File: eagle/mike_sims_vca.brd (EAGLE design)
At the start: 100 x 80 mm, 33 parts, among them IC2 LM13700N, IC3 TL072P, Q1 2N3906

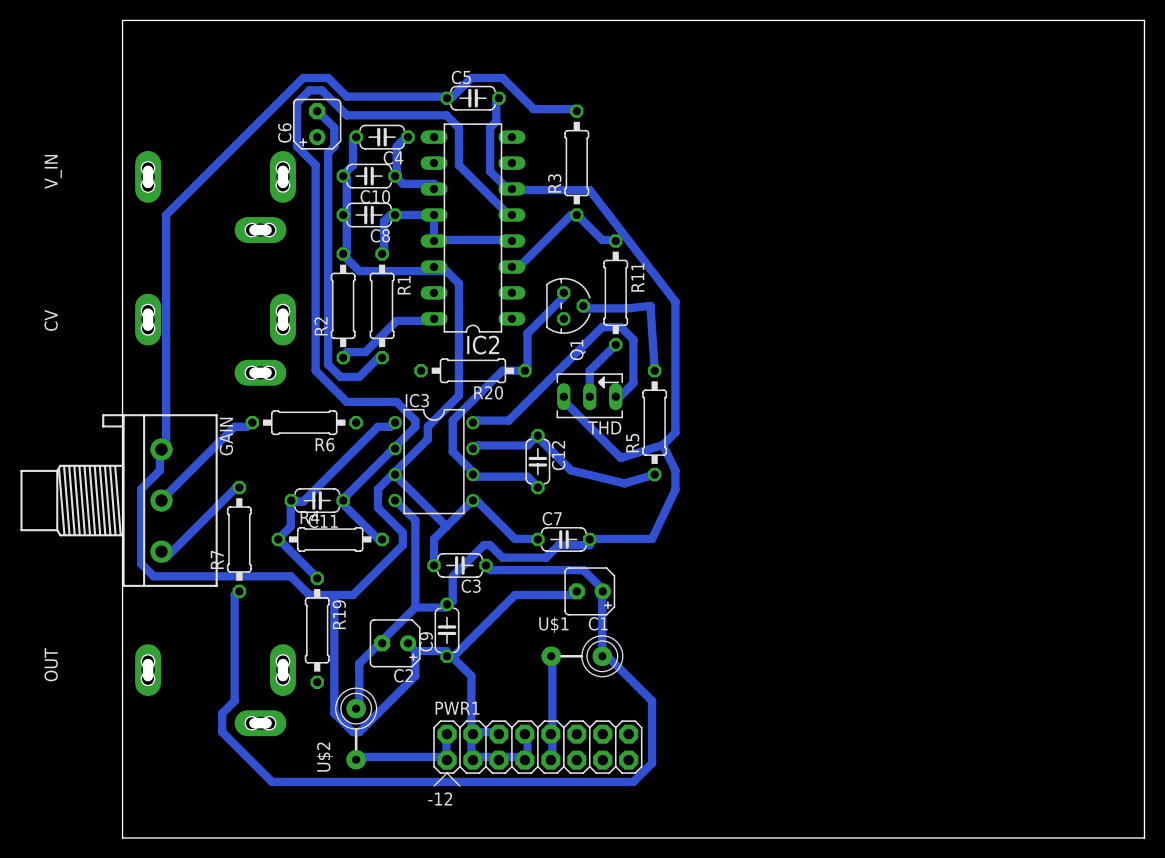
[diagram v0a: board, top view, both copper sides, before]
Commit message: routed
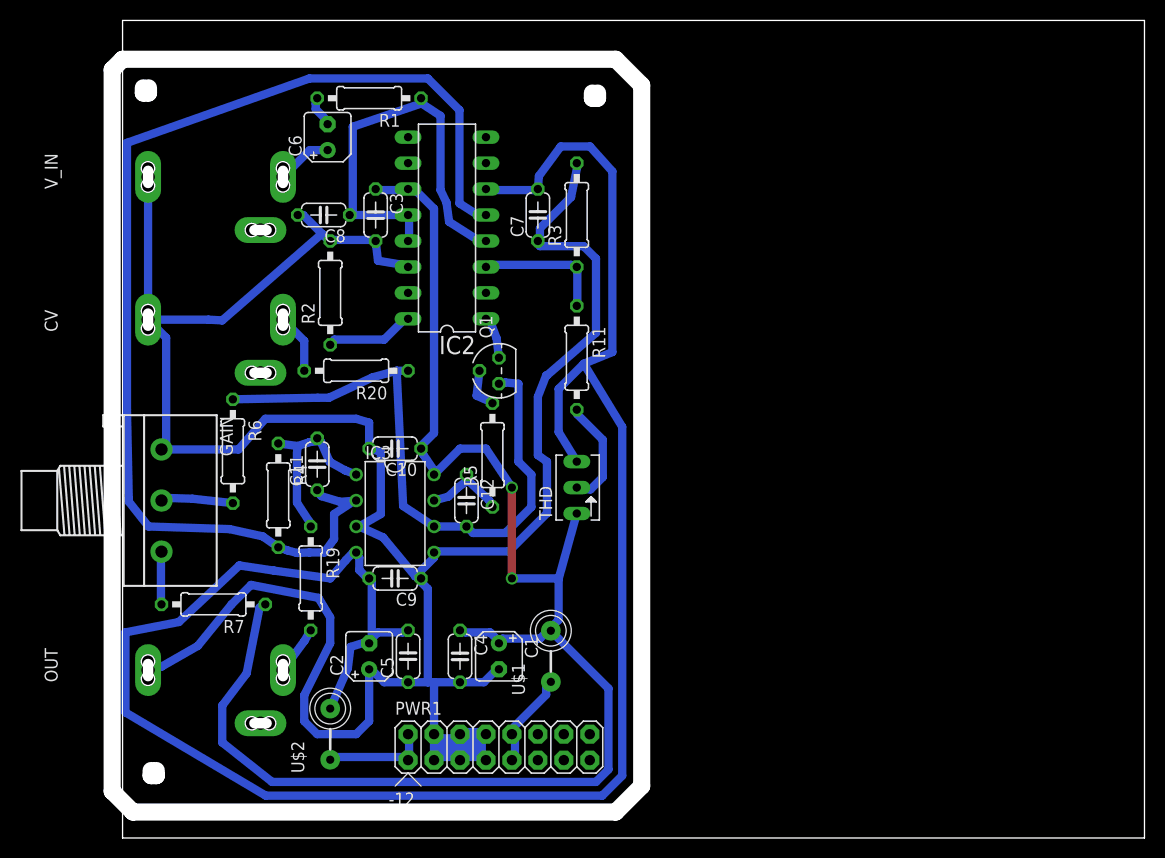
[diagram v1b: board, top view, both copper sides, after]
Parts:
- moved C5 55.0 mm to (27.9, 17.8), turned to 90 degrees
- moved C4 51.4 mm to (33.0, 17.8), turned to 270 degrees
- moved C3 35.3 mm to (24.8, 61.0), turned to 270 degrees
- moved C7 31.9 mm to (40.6, 61.0), turned to 90 degrees
- moved C10 26.8 mm to (26.7, 38.1)
- moved R1 20.4 mm to (24.1, 72.4), turned to 180 degrees
- moved R5 16.2 mm to (36.2, 37.5)
- moved R20 11.4 mm to (22.9, 45.7)
- moved C1 10.9 mm to (36.8, 17.8), turned to 270 degrees
- moved Q1 8.98 mm to (36.8, 45.7), turned to 90 degrees
- moved THD 8.98 mm to (44.5, 34.3), turned to 90 degrees
- moved C12 7.96 mm to (33.7, 33.0)
- moved R6 7.52 mm to (10.8, 37.8), turned to 270 degrees
- moved R11 7.41 mm to (44.5, 47.0)
- moved C9 7.18 mm to (26.7, 25.4), turned to 180 degrees
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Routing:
- net -12V: track 121.5 -> 196.6 mm
- net N$9: track 84.1 -> 114.0 mm
- net N$4: track 32.3 -> 3.07 mm
- net N$20: track 31.4 -> 59.9 mm
- net +12V: track 126.6 -> 149.9 mm, vias 0 -> 2
- net N$5: track 18.6 -> 41.5 mm
- net N$11: track 20.0 -> 8.24 mm
- net N$10: track 13.2 -> 4.24 mm
- net GND: track 258.1 -> 250.9 mm
- net N$25: track 0.00 -> 5.86 mm
- net N$13: track 10.7 -> 5.17 mm
- net N$3: track 0.00 -> 5.45 mm
- net N$8: track 23.1 -> 18.2 mm
- net N$24: track 0.00 -> 4.75 mm
- net N$19: track 6.13 -> 10.8 mm
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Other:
- board size 100 x 80 mm -> 101 x 80 mm
